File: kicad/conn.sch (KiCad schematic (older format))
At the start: 5 parts, among them J1701 NHD-4.3-480272FT-CTXL-T, J1702 NHD-4.3-480272FT-CTXL-T, J1703 NHD-4.3-480272FT-CTXL-T, J1704 tblock2x13, J1705 tblock2x13

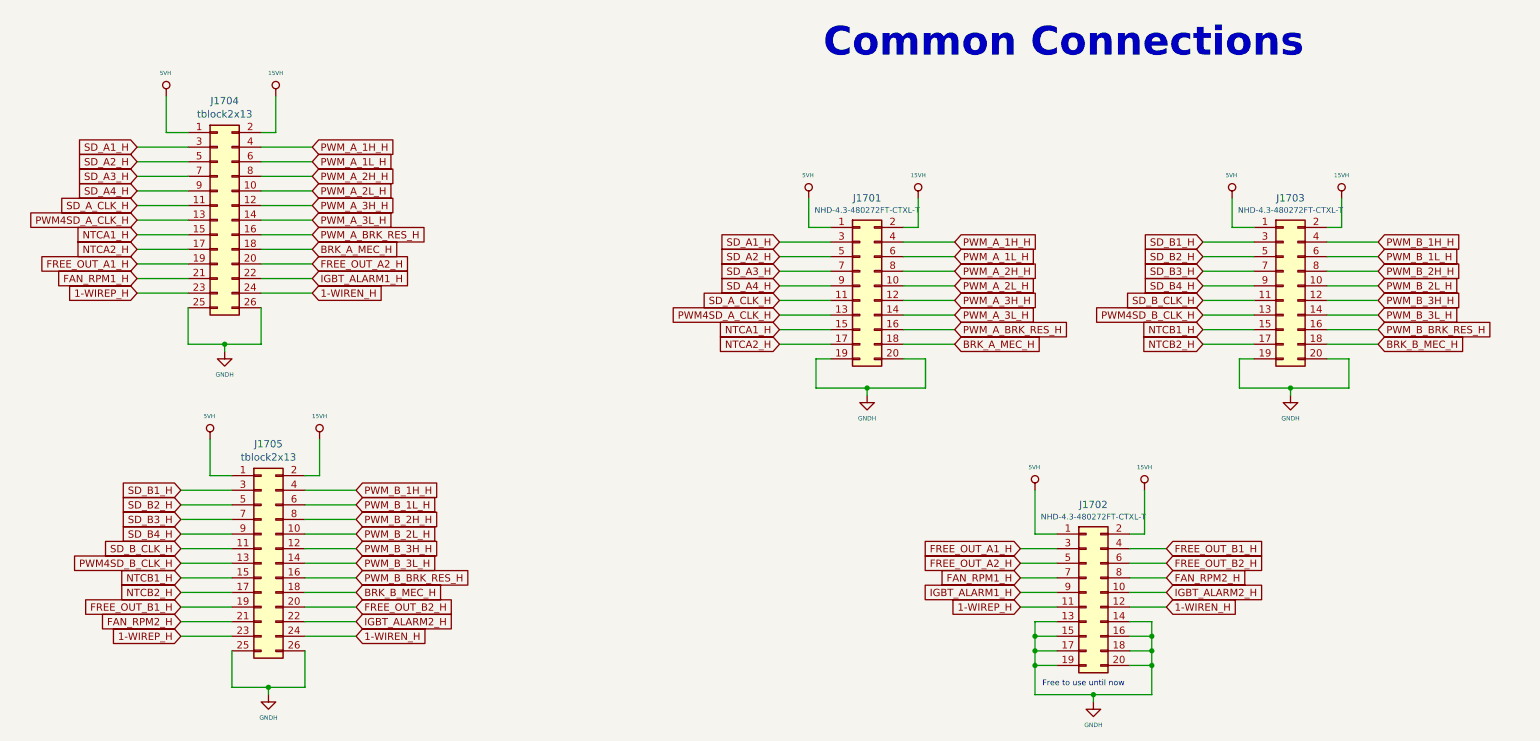
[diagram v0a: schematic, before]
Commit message: beginine routing... far far away
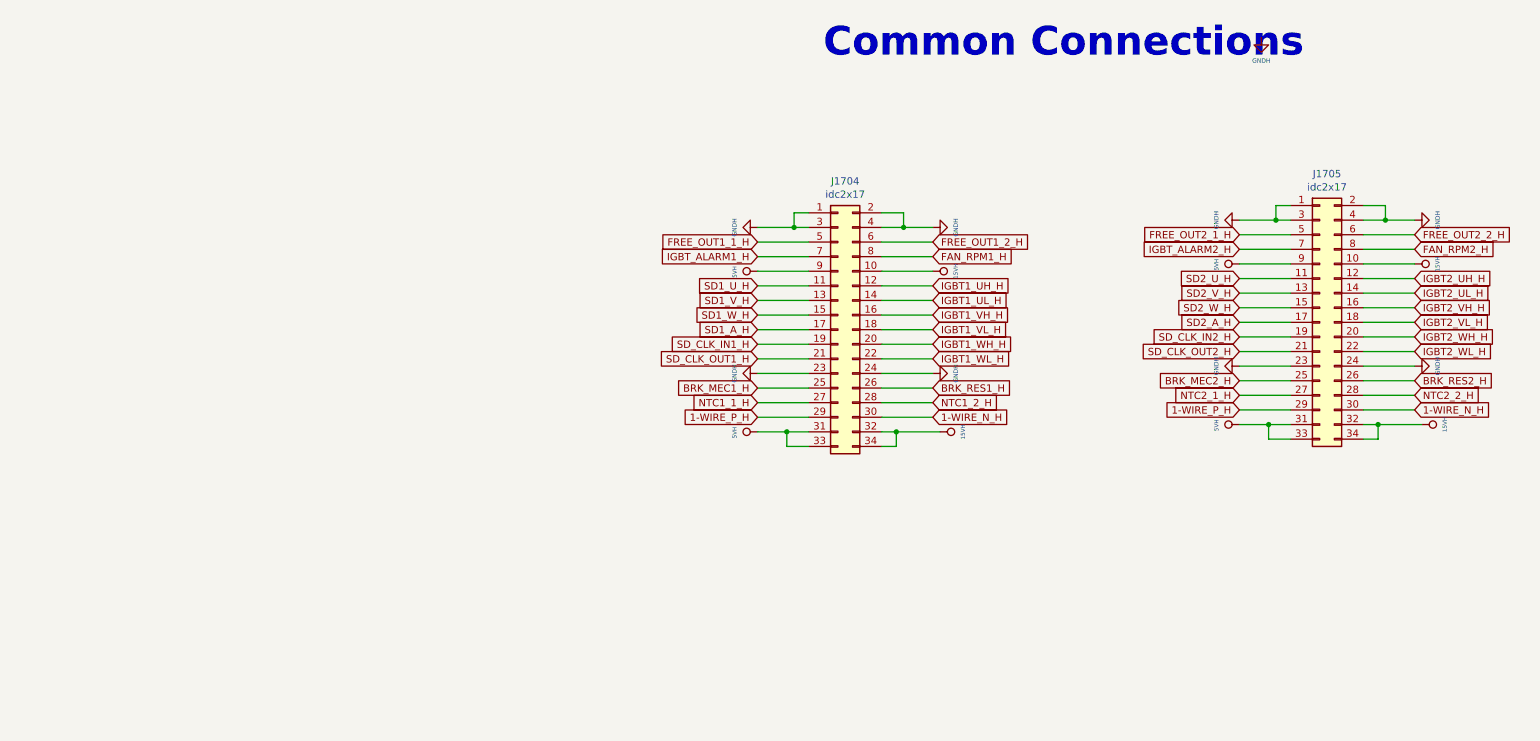
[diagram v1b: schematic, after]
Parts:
- removed J1701, J1702, J1703: NHD-4.3-480272FT-CTXL-T, Connector_IDC:IDC-Header_2x10_P2.54mm_Vertical, symbol servo:NHD-4.3-480272FT-CTXL-T
- removed J1704, J1705: tblock2x13, Connector_IDC:IDC-Header_2x13_P2.54mm_Vertical, symbol Connector_Generic:Conn_02x13_Odd_Even
- added J1704, J1705: idc2x17, servo:idc2x17_smd, symbol Connector_Generic:Conn_02x17_Odd_Even
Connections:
- net 15VH: now also J1704.10 (Pin_10), J1704.32 (Pin_32), J1704.34 (Pin_34), J1705.10 (Pin_10), J1705.32 (Pin_32), J1705.34 (Pin_34)
- net 5VH: now also J1704.31 (Pin_31), J1704.33 (Pin_33), J1704.9 (Pin_9), J1705.31 (Pin_31), J1705.33 (Pin_33), J1705.9 (Pin_9)
- net FAN_RPM1_H: now also J1704.8 (Pin_8)
- net FAN_RPM2_H: now also J1705.8 (Pin_8)
- net GNDH: now also J1704.1 (Pin_1), J1704.2 (Pin_2), J1704.23 (Pin_23), J1704.24 (Pin_24), J1704.3 (Pin_3), J1704.4 (Pin_4), J1705.1 (Pin_1), J1705.2 (Pin_2), J1705.23 (Pin_23), J1705.24 (Pin_24), J1705.3 (Pin_3), J1705.4 (Pin_4)
- net IGBT_ALARM1_H: now also J1704.7 (Pin_7)
- net IGBT_ALARM2_H: now also J1705.7 (Pin_7)
- new net 1-WIRE_N_H: J1704.30 (Pin_30), J1705.30 (Pin_30)
- new net 1-WIRE_P_H: J1704.29 (Pin_29), J1705.29 (Pin_29)
- new net BRK_MEC1_H: J1704.25 (Pin_25)
- new net BRK_MEC2_H: J1705.25 (Pin_25)
- new net BRK_RES1_H: J1704.26 (Pin_26)
- new net BRK_RES2_H: J1705.26 (Pin_26)
- new net FREE_OUT1_1_H: J1704.5 (Pin_5)
- new net FREE_OUT1_2_H: J1704.6 (Pin_6)
- new net FREE_OUT2_1_H: J1705.5 (Pin_5)
- new net FREE_OUT2_2_H: J1705.6 (Pin_6)
- new net IGBT1_UH_H: J1704.12 (Pin_12)
- new net IGBT1_UL_H: J1704.14 (Pin_14)
- new net IGBT1_VH_H: J1704.16 (Pin_16)
- new net IGBT1_VL_H: J1704.18 (Pin_18)
- new net IGBT1_WH_H: J1704.20 (Pin_20)
- new net IGBT1_WL_H: J1704.22 (Pin_22)
- new net IGBT2_UH_H: J1705.12 (Pin_12)
- new net IGBT2_UL_H: J1705.14 (Pin_14)
- new net IGBT2_VH_H: J1705.16 (Pin_16)
- new net IGBT2_VL_H: J1705.18 (Pin_18)
- new net IGBT2_WH_H: J1705.20 (Pin_20)
- new net IGBT2_WL_H: J1705.22 (Pin_22)
- new net NTC1_1_H: J1704.27 (Pin_27)
- new net NTC1_2_H: J1704.28 (Pin_28)
- new net NTC2_1_H: J1705.27 (Pin_27)
- new net NTC2_2_H: J1705.28 (Pin_28)
- new net SD1_A_H: J1704.17 (Pin_17)
- new net SD1_U_H: J1704.11 (Pin_11)
- new net SD1_V_H: J1704.13 (Pin_13)
- new net SD1_W_H: J1704.15 (Pin_15)
- new net SD2_A_H: J1705.17 (Pin_17)
- new net SD2_U_H: J1705.11 (Pin_11)
- new net SD2_V_H: J1705.13 (Pin_13)
- new net SD2_W_H: J1705.15 (Pin_15)
- new net SD_CLK_IN1_H: J1704.19 (Pin_19)
- new net SD_CLK_IN2_H: J1705.19 (Pin_19)
- new net SD_CLK_OUT1_H: J1704.21 (Pin_21)
- new net SD_CLK_OUT2_H: J1705.21 (Pin_21)
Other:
- note removed: "Free to use until now"
